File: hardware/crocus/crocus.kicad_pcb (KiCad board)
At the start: 4 copper layers, 70.7 x 53.3 mm, 49 parts, among them J1 NEIGHBOR1, J2 NEIGHBOR2, J7 BONUS_ROW, P1 RP-SMA, P2 EXPANSION, T1 BALUN, U1 nRF24L01+, U2 PCA9674, Y1 XTAL

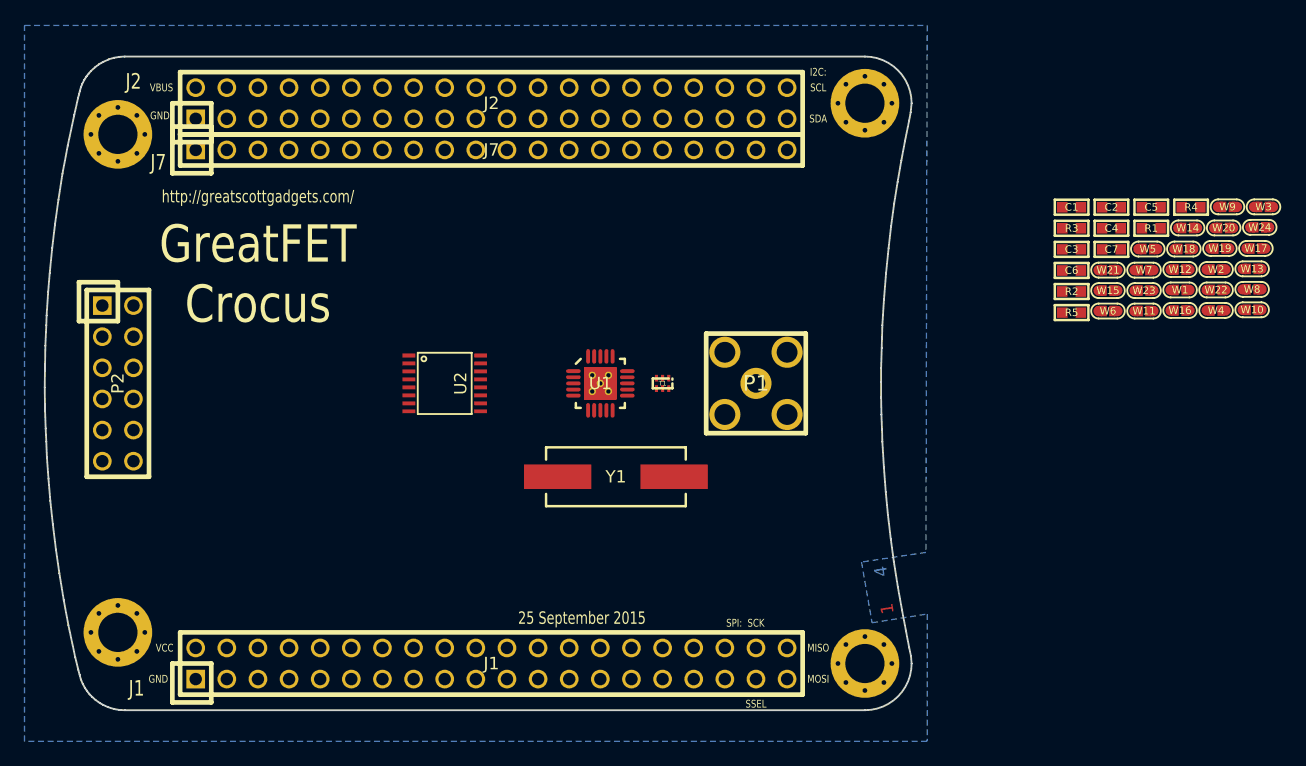
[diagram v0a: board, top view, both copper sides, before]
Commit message: crocus: finished layout
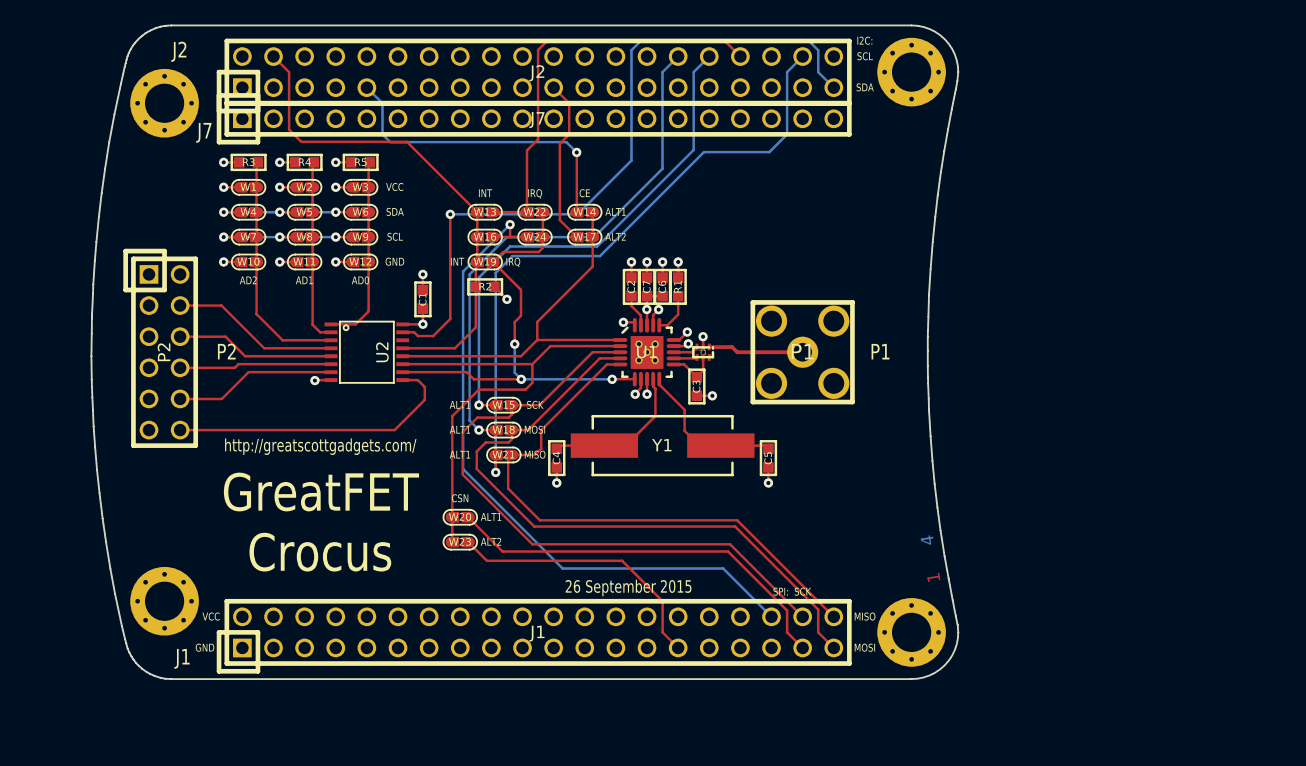
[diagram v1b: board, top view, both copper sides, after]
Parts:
- moved W10 82.0 mm to (122.4, 87.9)
- moved W4 79.4 mm to (122.4, 83.8)
- moved W8 77.4 mm to (127.0, 85.9)
- moved W1 76.5 mm to (122.4, 81.8)
- moved W2 74.7 mm to (127.0, 81.8)
- moved W3 73.7 mm to (131.6, 81.8)
- moved W7 73.1 mm to (122.4, 85.9)
- moved R4 72.4 mm to (127.0, 79.8), turned to 180 degrees
- moved W9 70.8 mm to (131.6, 85.9)
- moved W5 68.9 mm to (127.0, 83.8)
- moved W11 68.6 mm to (127.0, 87.9)
- moved R3 67.4 mm to (122.4, 79.8), turned to 180 degrees
- moved W12 66.9 mm to (131.6, 87.9)
- moved W20 66.6 mm to (139.7, 108.7), turned to 180 degrees
- moved W13 62.8 mm to (141.7, 83.8), turned to 180 degrees
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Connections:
- net /VBUS renamed Net-(J2-Pad2)
- net Net-(R3-Pad1) renamed /AD2
- net Net-(R4-Pad1) renamed /AD1
- net Net-(R5-Pad1) renamed /AD0
- J2 pad 1: GND -> Net-(J2-Pad1)
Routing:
- net /I2C0_SDA: track 0.00 -> 58.2 mm, vias 0 -> 1
- net /INT_ALT2: track 0.00 -> 55.6 mm, vias 0 -> 1
- net /MISO_ALT1: track 0.00 -> 53.0 mm, vias 0 -> 1
- net /MOSI: track 0.00 -> 53.0 mm
- net /SCK: track 0.00 -> 52.0 mm
- net /MISO: track 0.00 -> 46.4 mm
- net /MOSI_ALT1: track 0.00 -> 43.4 mm, vias 0 -> 1
- net /SCK_ALT1: track 0.00 -> 41.8 mm, vias 0 -> 1
- net /INT: track 0.00 -> 40.8 mm
- net /CSN: track 0.00 -> 37.8 mm
- net /IRQ: track 0.00 -> 37.6 mm, vias 0 -> 3
- net /INT_ALT1: track 0.00 -> 33.7 mm
- net /CSN_ALT1: track 0.00 -> 32.8 mm
- net /CE: track 0.00 -> 30.6 mm
- net /CE_ALT1: track 0.00 -> 25.7 mm, vias 0 -> 1
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- removed copper zone on B.Cu, net Net-(J2-Pad2)
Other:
- net class Default: clearance 0.1524 -> 0.2032
- rule trace_clearance: 0.1524 -> 0.2032
- board text added: "26 September 2015"
- board text added: "AD0"
- board text added: "AD1"
- board text added: "AD2"
- board text added: "ALT1"
- board text added: "ALT2"
- board text added: "CE"
- board text added: "CSN"
- board text added: "INT"
- board text added: "IRQ"
- board text added: "P1"
- board text added: "P2"
- board text removed: "25 September 2015"
- board text removed: "SSEL"
- board text removed: "VBUS"
